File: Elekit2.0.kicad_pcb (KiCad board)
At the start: 2 copper layers, 100 x 80 mm, 106 parts, among them J1 Screw_Terminal_01x02, J10 Conn_01x03_Male, J11 DS18B20 temperature sensor, J12 Conn_01x01_Male, J13 Conn_01x01_Male, J2 Screw_Terminal_01x02, J3 Screw_Terminal_01x02, J4 Screw_Terminal_01x02, J5 Conn_01x03_Male, J6 Conn_01x06_Male, J7 Conn_01x08, J8 Conn_01x08, J9 Conn_01x03_Male, Q1 2N7002, Q2 2N7002, Q3 2N7002, SW1 SW_Push, SW2 SW_Push, SW3 SW_Push, SW4 SW_Push, SW5 SW_Push, SW6 SW_Push, U1 MINI_5PTP, U10 TS-1187A-B-A-B, U11 DHT11, U12 DRV8870DDA, U15 DRV8870DDA, U2 MY-2032-12, U3 L7805, U4 MY-2032-12, U5 SRV05-4-P-T7, U6 74HC595, U7 ME6211C33M5G-N, U8 TS-1187A-B-A-B, U9 ESP32-C3-WROOM-02-N4(4MB)

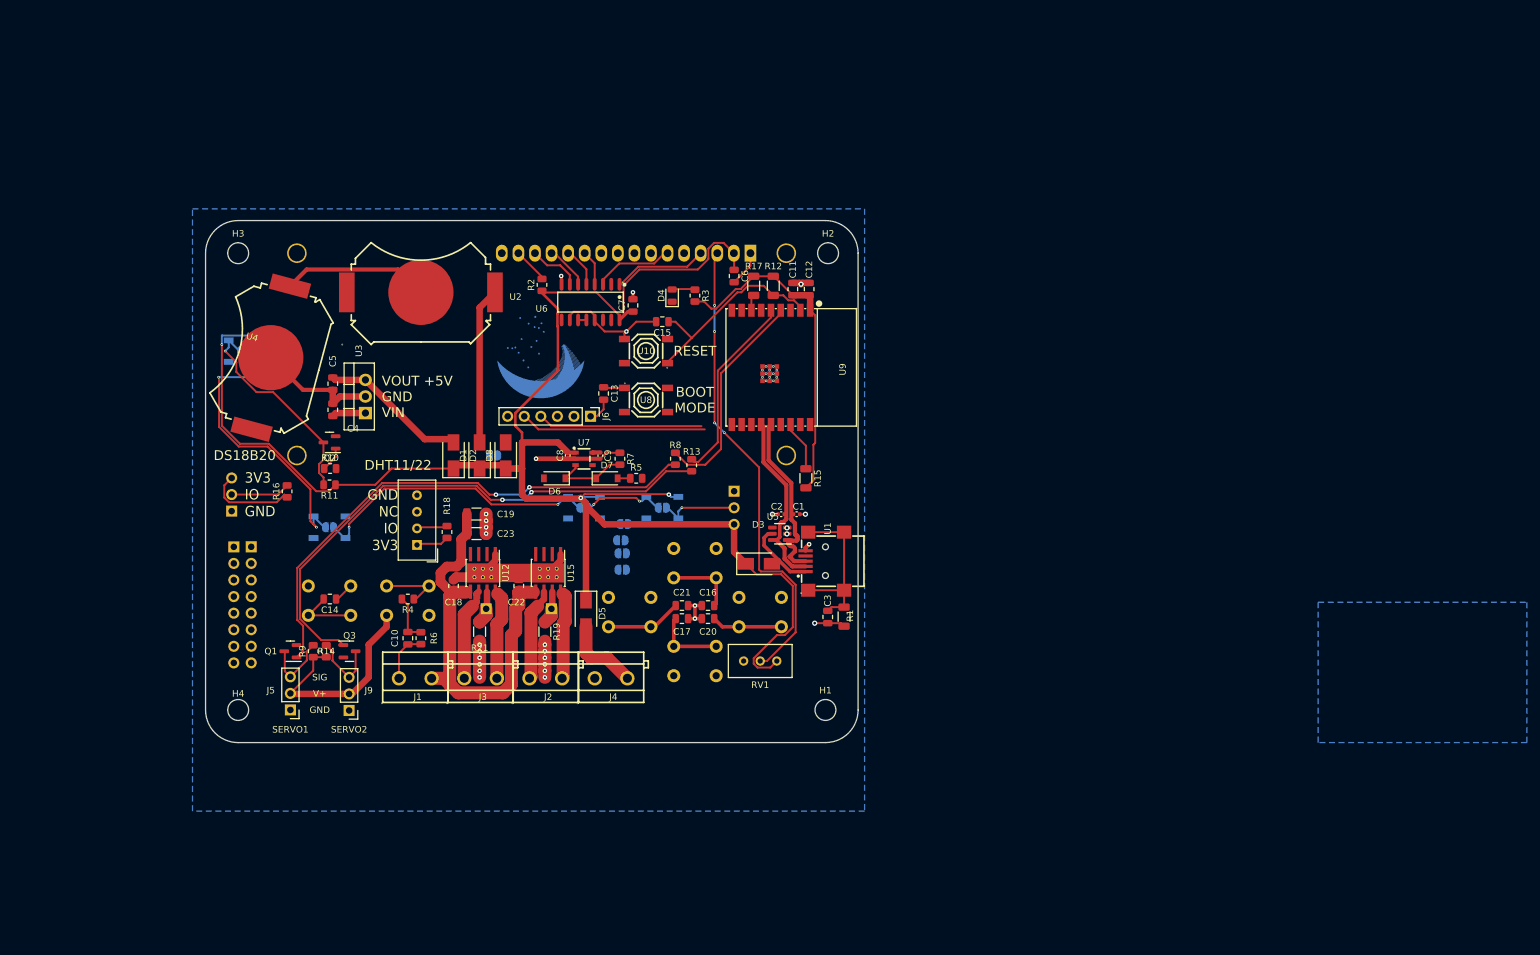
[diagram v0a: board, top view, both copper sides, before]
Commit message: Create first complete version
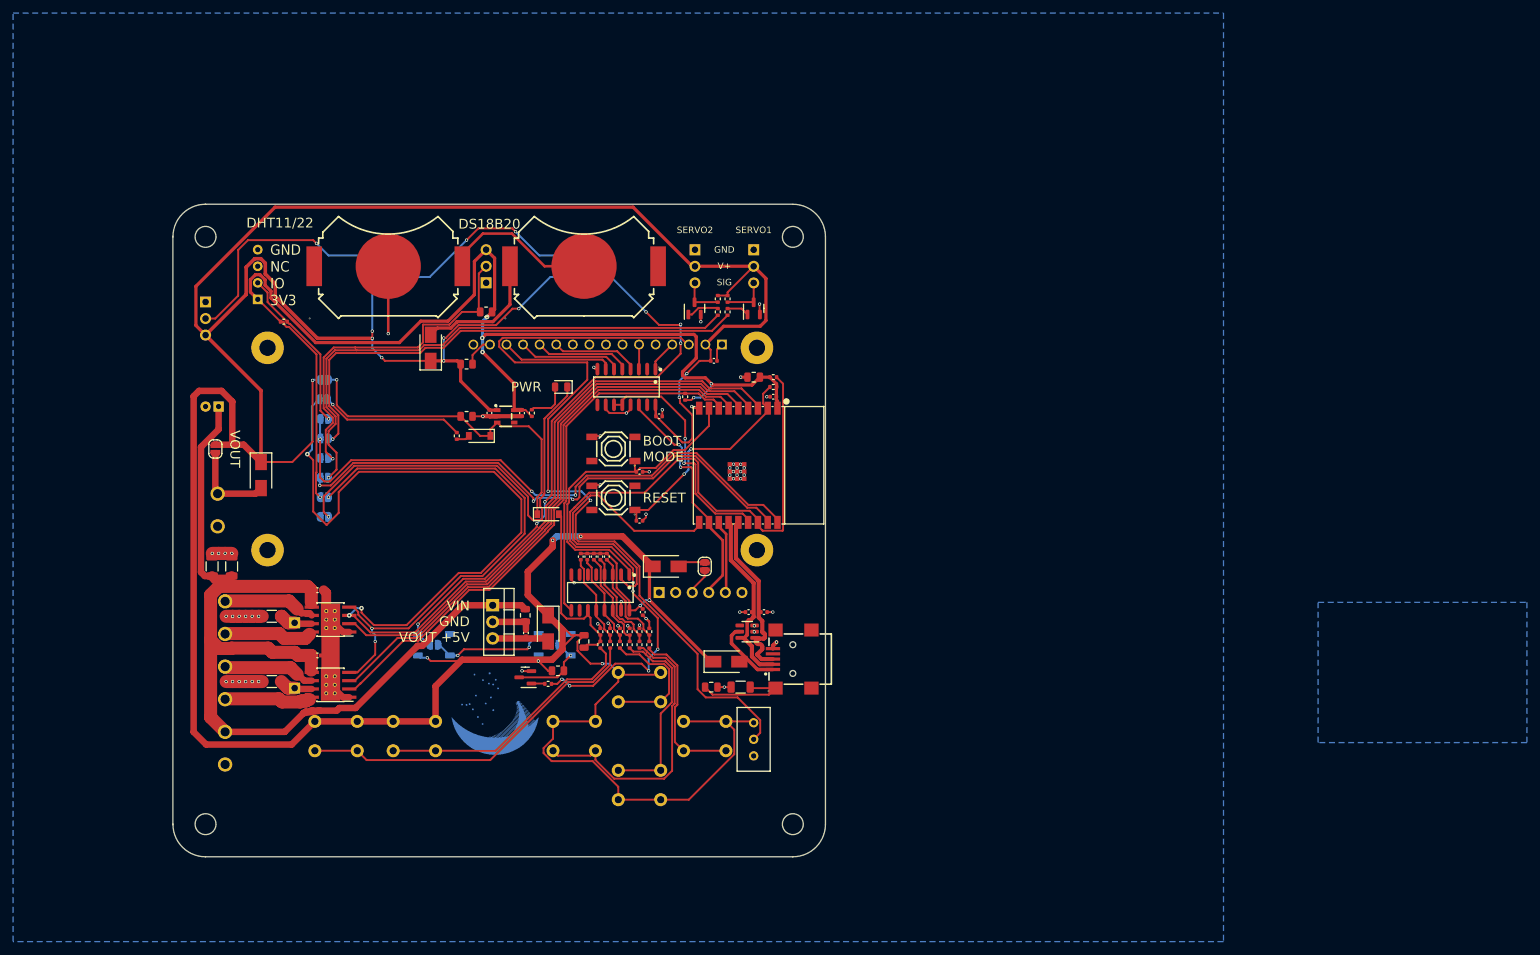
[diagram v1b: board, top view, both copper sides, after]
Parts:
- removed C10: 1u, Capacitor_SMD:C_0805_2012Metric
- removed J7, J8: Conn_01x08, Connector_PinHeader_2.54mm:PinHeader_1x08_P2.54mm_Vertical
- added C24: 0.1u 50V, Capacitor_SMD:C_0402_1005Metric, F.Cu at (80.5, 71.5)
- added C25: 1u, Capacitor_SMD:C_0805_2012Metric, F.Cu at (78.0, 84.5)
- added C26: C_Polarized, Capacitor_THT:CP_Radial_D5.0mm_P2.00mm, B.Cu at (22.0, 48.5)
- added JP10: Servo1, Jumper:SolderJumper-2_P1.3mm_Open_RoundedPad1.0x1.5mm, B.Cu at (38.2, 56.4)
- added JP11: Servo1, Jumper:SolderJumper-2_P1.3mm_Open_RoundedPad1.0x1.5mm, B.Cu at (38.2, 59.4)
- added JP12: Servo1, Jumper:SolderJumper-2_P1.3mm_Open_RoundedPad1.0x1.5mm, B.Cu at (38.2, 50.4)
- added JP13: Servo1, Jumper:SolderJumper-2_P1.3mm_Open_RoundedPad1.0x1.5mm, B.Cu at (38.2, 53.4)
- added JP14: Latch control, Jumper:SolderJumper-2_P1.3mm_Open_RoundedPad1.0x1.5mm, B.Cu at (38.0, 47.4)
- added R20: 1k, Resistor_SMD:R_0402_1005Metric, F.Cu at (82.0, 85.0)
- added R22: 10k, Resistor_SMD:R_0402_1005Metric, F.Cu at (82.0, 83.0)
- added R23: 1k, Resistor_SMD:R_0402_1005Metric, F.Cu at (83.5, 85.0)
- added R24: 1k, Resistor_SMD:R_0402_1005Metric, F.Cu at (85.0, 85.0)
- added R25: 1k, Resistor_SMD:R_0402_1005Metric, F.Cu at (88.0, 85.0)
- added R26: 1k, Resistor_SMD:R_0402_1005Metric, F.Cu at (86.5, 85.0)
- added R28: 10k, Resistor_SMD:R_0402_1005Metric, F.Cu at (83.5, 83.0)
- added R29: 10k, Resistor_SMD:R_0402_1005Metric, F.Cu at (85.0, 83.0)
- added R30: 10k, Resistor_SMD:R_0402_1005Metric, F.Cu at (88.0, 83.0)
- added R33: 10k, Resistor_SMD:R_0402_1005Metric, F.Cu at (86.5, 83.0)
- added U13: 74HC165, 0_JLCPCB_Footprints:SOIC-16_L9.9-W3.9-P1.27-LS6.0-BL, F.Cu at (80.5, 77.0)
- C12, C13, C14, C15, C16, C17, C18, C20, C21, C22, C5, C6, C7: value 0.1u -> 0.1u 50V; footprint Capacitor_SMD:C_0805_2012Metric -> Capacitor_SMD:C_0402_1005Metric
- DS1: footprint Display:WC1602A -> SnapEDA Library:LCD_RC1602B-BIW-CSV
- J1, J2, J3, J4, J5, J6, J9, U11: moved to B.Cu
- J12: footprint Connector_PinHeader_2.54mm:PinHeader_1x01_P2.54mm_Vertical -> 0_JLCPCB_Footprints:PinHeader_1x01_P2.54mm_Vertical
- JP2, JP5: moved to F.Cu
- JP3: value Latch control -> H-Bridge
- JP4: value Power LED -> PWR LED
- R10, R13, R14, R18, R3, R5, R6, R8, R9: footprint Resistor_SMD:R_0805_2012Metric -> Resistor_SMD:R_0402_1005Metric
- R12, R15, R17: footprint Resistor_SMD:R_1206_3216Metric -> Resistor_SMD:R_0402_1005Metric
- R4: value 10k -> 1k; footprint Resistor_SMD:R_0805_2012Metric -> Resistor_SMD:R_0402_1005Metric
- moved J5 100.1 mm to (104.0, 24.5)
- moved Q1 88.3 mm to (104.0, 33.5), turned to 90 degrees
- moved J9 88.3 mm to (95.0, 24.5)
- moved J10 86.0 mm to (20.0, 32.5)
- moved R9 83.4 mm to (100.0, 32.0), turned to -90 degrees
- moved R14 80.7 mm to (98.5, 32.0), turned to -90 degrees
- moved Q3 74.5 mm to (94.9, 33.5), turned to 90 degrees
- moved J4 65.9 mm to (22.0, 64.0), turned to 90 degrees
- moved JP2 64.4 mm to (21.5, 55.0), turned to -90 degrees
- moved LOGO1 55.1 mm to (71.5, 88.0)
- moved JP1 54.1 mm to (38.2, 44.4)
- moved D5 54.1 mm to (28.5, 59.0)
- moved D11 53.6 mm to (78.0, 27.0), turned to 0 degrees
- moved JP8 53.6 mm to (78.0, 27.0), turned to 180 degrees
- moved J11 52.4 mm to (63.0, 29.5)
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- renumbered D12 to D10, D9 to D11, D10 to D12, D11 to D9, JP8 to JP6, JP9 to JP7, JP6 to JP8, JP7 to JP9
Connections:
- net /BTN renamed /BTN1
- C14 pad 1: GND -> /VBUS
- C14 pad 2: Net-(C14-Pad2) -> GND
- C16 pad 1: GND -> /BTN2
- C16 pad 2: Net-(C16-Pad2) -> /VBUS
- C17 pad 1: GND -> /BTN3
- C17 pad 2: Net-(C17-Pad2) -> /VBUS
- C20 pad 1: GND -> /BTN4
- C20 pad 2: Net-(C20-Pad2) -> /VBUS
- C21 pad 1: GND -> /BTN5
- C21 pad 2: Net-(C21-Pad2) -> /VBUS
- D10 pad 2: Net-(D12-Pad2) -> Net-(D10-Pad2)
- D11 pad 4: Net-(D9-Pad4) -> Net-(D10-Pad2)
- D12 pad 2: Net-(D10-Pad2) -> Net-(D12-Pad2)
- D9 pad 4: Net-(D10-Pad2) -> Net-(D9-Pad4)
- J2 pad 1: /A1 -> /A2
- J2 pad 2: /A2 -> /A1
- J3 pad 1: /B1 -> /B2
- J3 pad 2: /B2 -> /B1
- JP3 pad 1: Net-(JP3-Pad1) -> +3.3V
- JP3 pad 2: /GPIO4 -> /H-BRIDGE_PWR
- JP6 pad 1: Net-(D10-Pad2) -> Net-(D9-Pad4)
- JP7 pad 2: Net-(D12-Pad2) -> Net-(D10-Pad2)
- JP8 pad 1: Net-(D9-Pad4) -> Net-(D10-Pad2)
- JP9 pad 2: Net-(D10-Pad2) -> Net-(D12-Pad2)
- R10 pad 2: /GPIO5 -> /GPIO2
- R13 pad 2: /GPIO6 -> /SERVO2_c
- R5 pad 2: Net-(JP3-Pad1) -> /Latch control
- R8 pad 2: /GPIO5 -> /SERVO1_c
- SW2 pad 1: GND -> /VBUS
- SW2 pad 2: Net-(C14-Pad2) -> Net-(R20-Pad1)
- SW3 pad 1: GND -> /VBUS
- SW3 pad 2: Net-(C16-Pad2) -> Net-(R23-Pad1)
- SW4 pad 1: GND -> /VBUS
- SW4 pad 2: Net-(C17-Pad2) -> Net-(R24-Pad1)
- SW5 pad 1: GND -> /VBUS
- SW5 pad 2: Net-(C20-Pad2) -> Net-(R25-Pad1)
- SW6 pad 1: GND -> /VBUS
- SW6 pad 2: Net-(C21-Pad2) -> Net-(R26-Pad1)
- U12 pad 4: +3.3V -> /H-BRIDGE_PWR
- U15 pad 4: +3.3V -> /H-BRIDGE_PWR
- U6 pad 11: Net-(U6-Pad11) -> /CLK2
- U6 pad 12: Net-(U6-Pad11) -> /CLK2
- U6 pad 14: unconnected-(U6-Pad14) -> /RX
- U9 pad 10: /GPIO10 -> /CLK1
- U9 pad 15: /GPIO3 -> /CLK2
- U9 pad 3: /GPIO4 -> /B1_c
- U9 pad 4: /GPIO5 -> /B2_C
- U9 pad 5: /GPIO6 -> /A1_c
- U9 pad 6: /GPIO7 -> /A2_C
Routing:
- net /VBUS: track 297.8 -> 648.2 mm, vias 3 -> 17
- net /B1_c: track 0.00 -> 187.2 mm, vias 0 -> 3
- net +3.3V: track 72.0 -> 185.2 mm, vias 0 -> 6
- net /GPIO2: track 7.76 -> 118.9 mm, vias 0 -> 6
- net /GPIO0: track 0.00 -> 90.9 mm, vias 0 -> 3
- net /A1_c: track 0.00 -> 88.1 mm
- net /B2_C: track 0.00 -> 87.8 mm
- net /A2_C: track 0.00 -> 86.7 mm
- net /GPIO1: track 0.00 -> 85.5 mm, vias 0 -> 3
- net /H-BRIDGE_PWR: track 0.00 -> 83.0 mm, vias 0 -> 3
- net /SERVO2_c: track 0.00 -> 83.0 mm, vias 0 -> 1
- net /HVBUS: track 67.6 -> 147.4 mm
- net Net-(Q3-Pad1): track 84.6 -> 4.98 mm, vias 2 -> 0
- net /SERVO1_c: track 0.00 -> 77.7 mm, vias 0 -> 1
- net Net-(Q1-Pad1): track 80.6 -> 3.43 mm, vias 2 -> 0
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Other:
- board size 100 x 80 mm -> 100 x 100 mm
- board text added: "A1"
- board text added: "A2"
- board text added: "B1"
- board text added: "B2"
- board text added: "Constant PWR"
- board text added: "H-Bridge PWR"
- board text added: "IO0"
- board text added: "IO1"
- board text added: "IO4"
- board text added: "PWR"
- board text added: "PWR LED"
- board text added: "PWR Latch"
- board text added: "VIN"
- board text added: "VIN 5-6V"
- board text added: "VIN GND VOUT +5V"
- board text added: "VOUT"
- board text removed: "VOUT +5V GND VIN"
